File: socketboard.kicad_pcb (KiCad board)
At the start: 2 copper layers, 22.5 x 57 mm, 12 parts, among them J1 GPIO, J2 Conn_01x07, J3 Conn_01x03, U1 MCP2518FDT-H/SL, U2 ATA6563-GBQW1, Y1 Oscillator

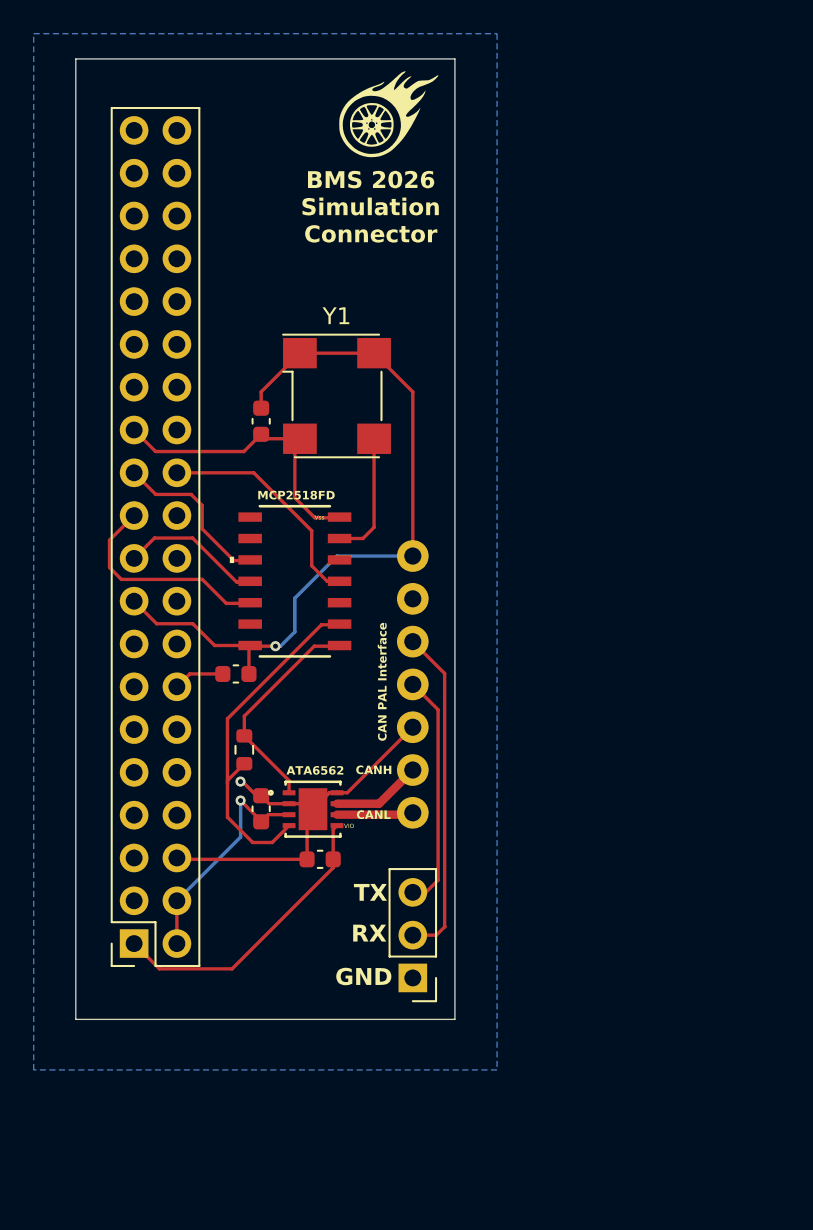
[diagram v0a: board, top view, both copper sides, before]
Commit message: final
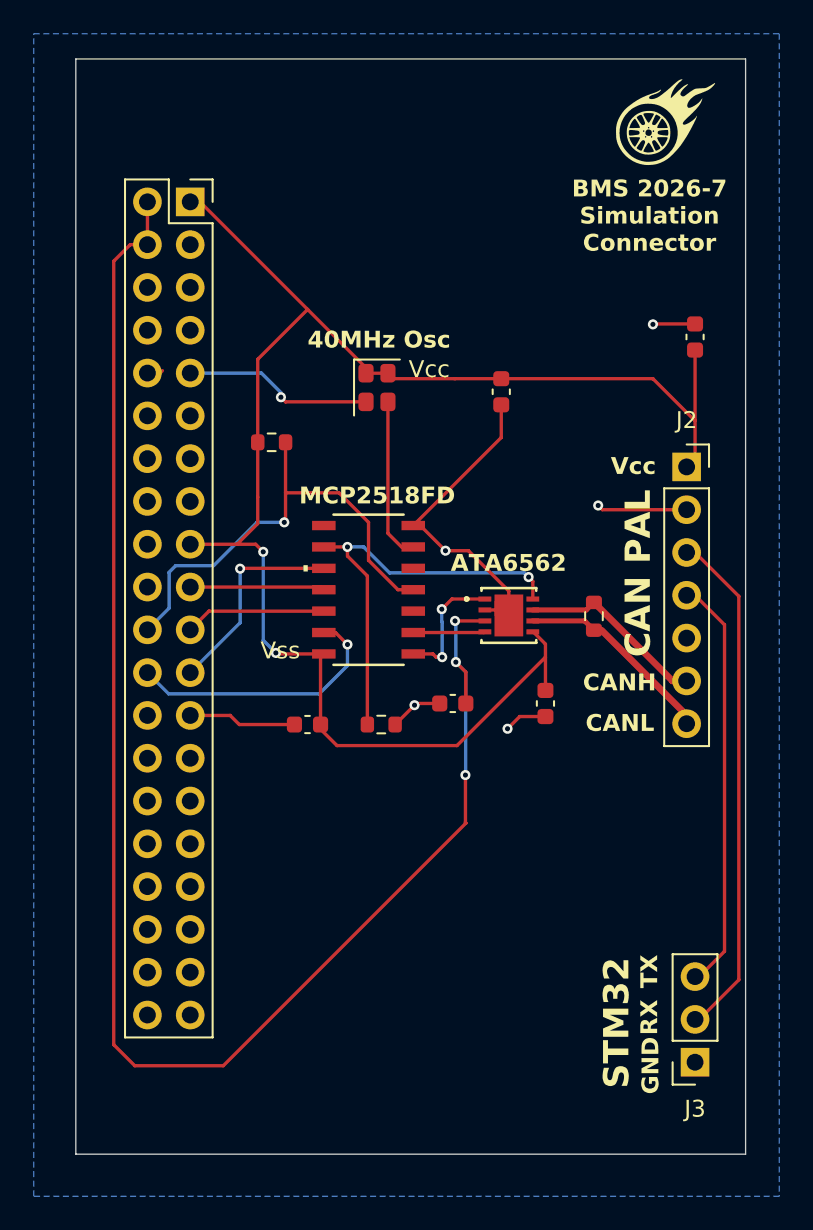
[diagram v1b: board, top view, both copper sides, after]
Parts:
- removed Y1: Oscillator, Oscillator:Oscillator_SMD_Diodes_FN-4Pin_7.0x5.0mm
- added C5: 4.7uF, PCM_SparkFun-Capacitor:C_0603_1608Metric, F.Cu at (71.8, 61.5)
- added R2: 10k, PCM_SparkFun-Resistor:R_0603_1608Metric, F.Cu at (46.6, 67.8)
- added R3: 4.7k, PCM_SparkFun-Resistor:R_0603_1608Metric, F.Cu at (53.1, 84.5)
- added Y2: SG-210STF, Oscillator:Oscillator_SMD_SeikoEpson_SG210-4Pin_2.5x2.0mm, F.Cu at (52.9, 64.5)
- J2: footprint PCM_SparkFun-Connector:1x07_P2.54mm -> Connector_PinSocket_2.54mm:PinSocket_1x07_P2.54mm_Vertical
- J3: footprint Connector_PinHeader_2.54mm:PinHeader_1x03_P2.54mm_Vertical -> Connector_PinSocket_2.54mm:PinSocket_1x03_P2.54mm_Vertical
- moved J1 44.1 mm to (41.8, 53.5), turned to 0 degrees
- moved R1 22.2 mm to (65.8, 78.1), turned to 90 degrees
- moved J3 17.5 mm to (71.8, 104.5)
- moved J2 17.1 mm to (71.2, 69.2), turned to 0 degrees
- moved G*** 16.4 mm to (70.4, 48.5)
- moved U2 16.4 mm to (60.7, 78.0)
- moved C4 16.3 mm to (62.9, 83.2), turned to 90 degrees
- moved C1 14.4 mm to (60.2, 64.8), turned to 90 degrees
- moved C3 13.0 mm to (57.4, 83.2), turned to 180 degrees
- moved C2 5.20 mm to (48.8, 84.5)
- moved U1 4.40 mm to (52.4, 76.5)
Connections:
- C1 pad 1: 3.3V -> GND
- C1 pad 2: GND -> 3.3V
- J1 pad 22: unconnected-(J1-Pin_22-Pad22) -> /GPIO25
- R1 pad 1: /TXD -> /CANL
- R1 pad 2: /RXD -> /CANH
- U1 pad 13: unconnected-(U1-NCS-Pad13) -> /GPIO8/SPI0.CE0
- U1 pad 4: /GPIO8/SPI0.CE0 -> /GPIO25
- U1 pad 9: unconnected-(U1-*INT0/GPIO0/XSTBY-Pad9) -> /STBY
- U2 pad 8: GND -> /STBY
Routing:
- net 5V: track 13.7 -> 95.6 mm, vias 1 -> 3
- net 3.3V: track 62.1 -> 96.0 mm, vias 1 -> 2
- net /GPIO25: track 0.00 -> 28.3 mm, vias 0 -> 1
- net /STBY: track 0.00 -> 25.3 mm, vias 0 -> 2
- net /RXD: track 20.4 -> 4.69 mm
- net /RX_MCU: track 19.8 -> 29.8 mm
- net /TX_MCU: track 14.0 -> 24.0 mm
- net /CANL: track 4.55 -> 12.2 mm
- net GND: track 44.2 -> 51.2 mm, vias 1 -> 6
- net /CANH: track 5.33 -> 11.7 mm
- net /TXD: track 12.4 -> 7.46 mm, vias 0 -> 2
- net /GPIO9/SPI0.MISO: track 12.3 -> 8.39 mm
- net /GPIO11/SPI0.SCLK: track 9.20 -> 12.4 mm, vias 0 -> 1
- net /GPIO8/SPI0.CE0: track 13.5 -> 16.0 mm, vias 0 -> 1
- net /OSC1: track 7.58 -> 9.64 mm
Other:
- board size 22.5 x 57 mm -> 39.8 x 65 mm
- board text added: "40MHz Osc"
- board text added: "BMS 2026-7 Simulation Connector"
- board text added: "CAN PAL"
- board text added: "STM32"
- board text added: "Vcc"
- board text removed: "BMS 2026 Simulation Connector"
- board text removed: "CAN PAL Interface"
- board text removed: "VIO"
